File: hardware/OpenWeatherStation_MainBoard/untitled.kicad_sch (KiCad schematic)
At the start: 50 parts, among them Q1 Q_NMOS_GDS, U5 PM8800A, U6 POE13P-33L

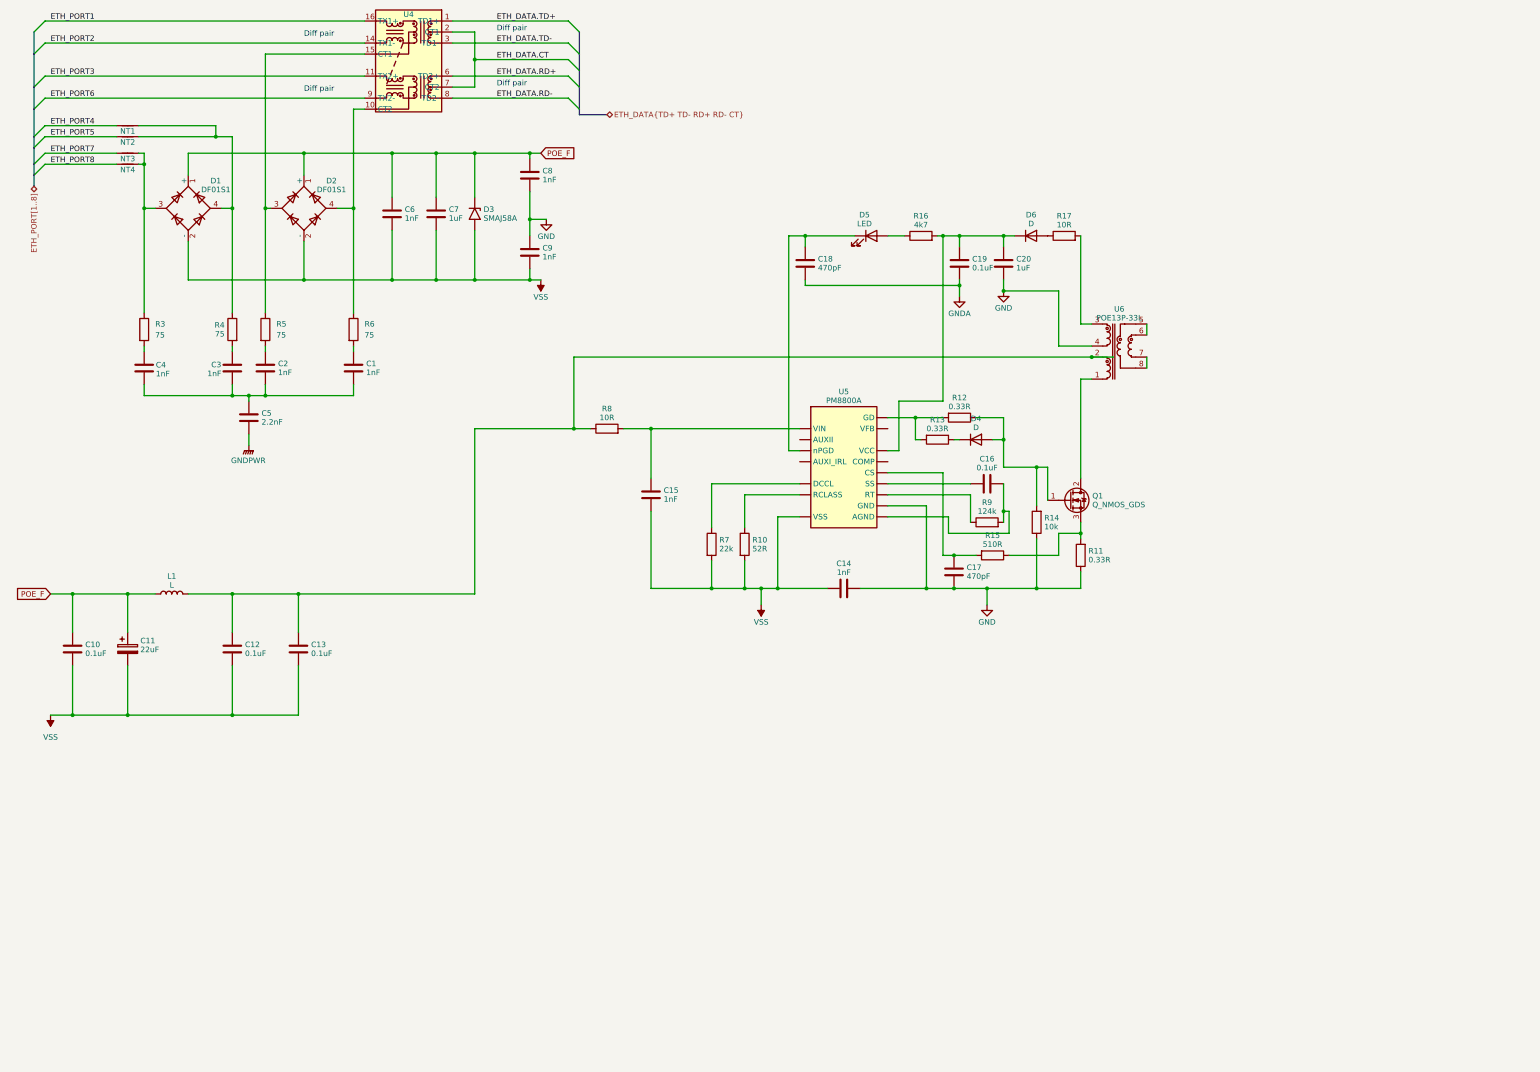
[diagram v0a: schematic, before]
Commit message: poe wip
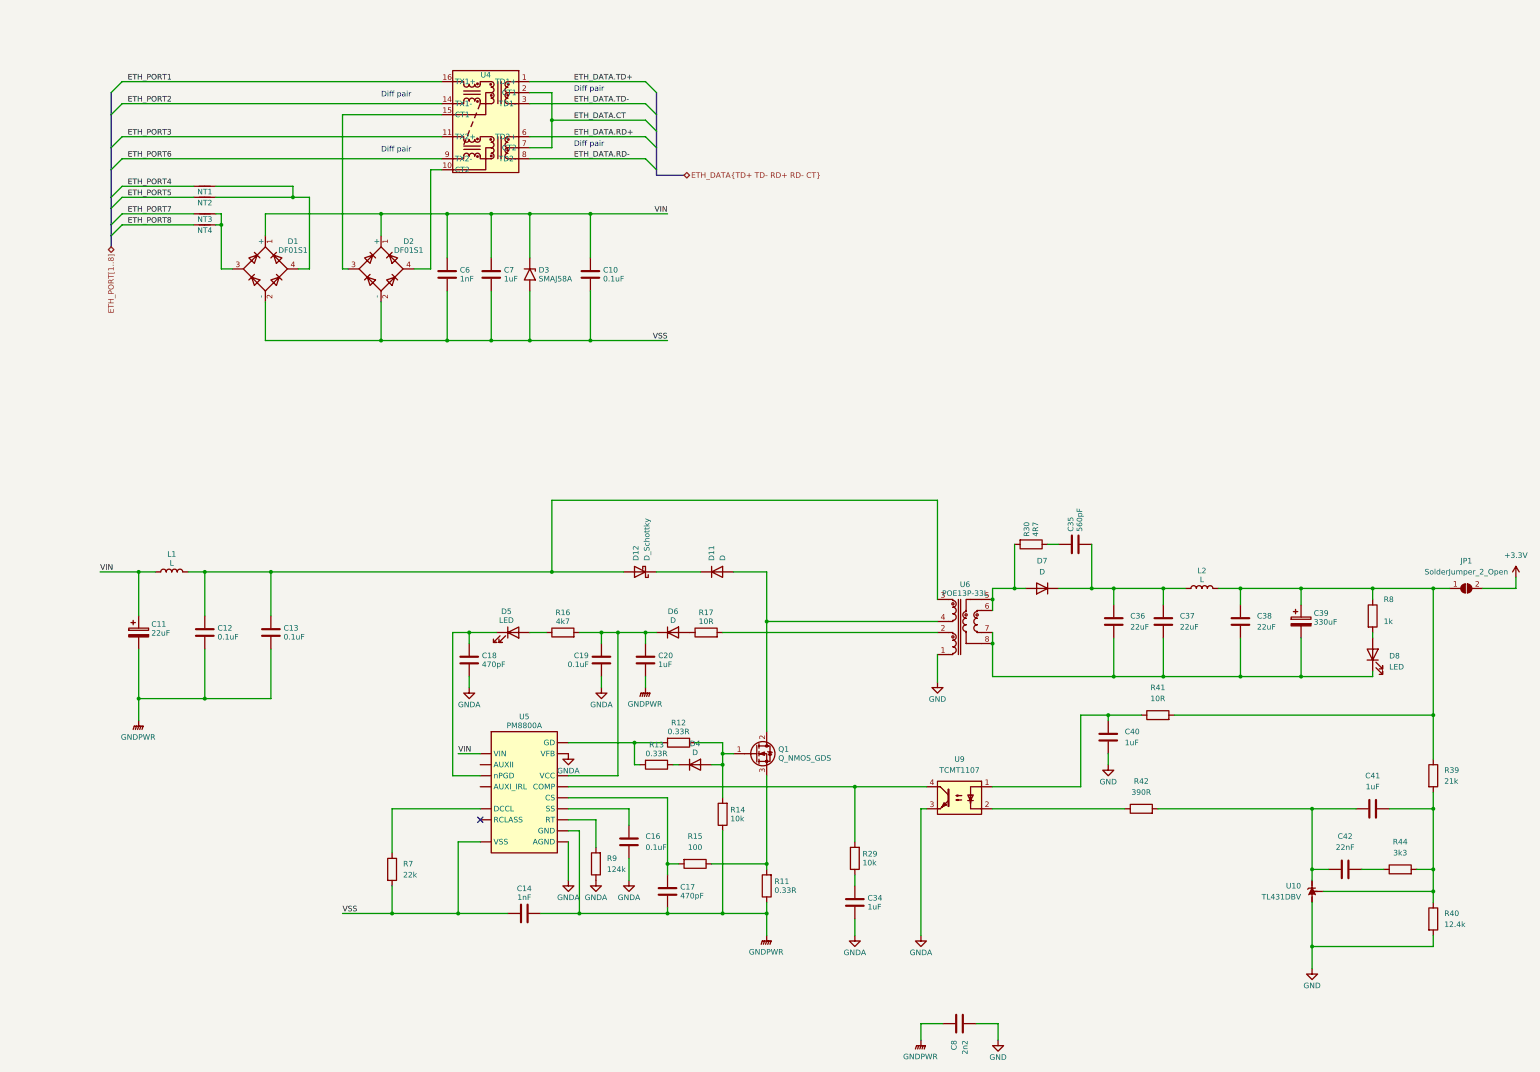
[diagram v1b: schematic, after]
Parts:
- removed C1, C15, C2, C3, C4, C9: 1nF, symbol Device:C
- removed C5: 2.2nF, symbol Device:C
- removed R10: 52R, symbol Device:R
- removed R3, R4, R5, R6: 75, symbol Device:R
- added C34, C40, C41: 1uF, symbol Device:C
- added C35: 560pF, symbol Device:C
- added C36, C37, C38: 22uF, symbol Device:C
- added C39: 330uF, symbol Device:C_Polarized
- added C42: 22nF, symbol Device:C
- added D11, D7: D, symbol Device:D
- added D12: D_Schottky, symbol Device:D_Schottky
- added D8: LED, symbol Device:LED
- added JP1: SolderJumper_2_Open, symbol Jumper:SolderJumper_2_Open
- added L2: L, symbol Device:L
- added R29: 10k, symbol Device:R
- added R30: 4R7, Resistor_SMD:R_1206_3216Metric, symbol Device:R
- added R39: 21k, symbol Device:R
- added R40: 12.4k, symbol Device:R
- added R41: 10R, symbol Device:R
- added R42: 390R, symbol Device:R
- added R44: 3k3, symbol Device:R
- added U10: TL431DBV, Package_TO_SOT_SMD:SOT-23-5, symbol Reference_Voltage:TL431DBV
- added U9: TCMT1107, Package_SO:SOP-4_4.4x2.6mm_P1.27mm, symbol Isolator:TCMT1107
- C8: value 1nF -> 2n2
- R15: value 510R -> 100
- R8: value 10R -> 1k
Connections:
- net GND: now also U6.1, C40.1, R40.2, U10.5 (A); no longer C14.2, C17.2, C20.2, R11.1, R14.1, U5. (nPGD), U6.4
- net GNDA: now also C16.2, R9.1, U5. (nPGD), C34.2, U9.3
- net GNDPWR: now also C11.2, C12.2, C13.2, C14.2, C17.2, C20.2, C8.1, R11.1, R14.1, U5. (nPGD)
- net VSS: no longer C11.2, C12.2, C13.2
- net at C12.1, C13.1, L1.2: now also U6.3, D12.2 (A); no longer R8.1, U6.2
- net at R8.2: now also D8.2 (A); no longer U5. (nPGD)
- net at Q1.2 (D): now also U6.4, D11.2 (A); no longer U6.1
- net at R17.2: now also U6.2; no longer U6.3
- net at U6.5, U6.6: now also D7.2 (A), R30.2
- net at U6.7, U6.8: now also C36.1, C37.1, C38.1, C39.2, D8.1 (K)
- net POE_F renamed VIN
- net VIN: now also U5. (nPGD); no longer C8.1
- new net: D11.1 (K), D12.1 (K)
- new net: R9.2, U5. (nPGD)
- new net: C41.1, R39.2, R40.1, R44.2, U10.4 (REF)
- new net: C40.2, R41.1, U9.1
- new net: C38.2, C39.1, JP1.1 (A), L2.2, R39.1, R41.2, R8.1
- new net: C34.1, R29.1
- new net: R29.2, U5. (nPGD), U9.4
- new net: R42.1, U9.2
- new net: C35.1, R30.1
- new net: C35.2, C36.2, C37.2, D7.1 (K), L2.1
- new net: C42.1, R44.1
- new net: C41.2, C42.2, R42.2, U10.3 (K)
- new net: C16.1, U5. (nPGD)
- new net +3.3V: JP1.2 (B)
- no-connect marks 0 -> 1
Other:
- moved on the sheet: C10, C11, C12, C13, C14, C16, C17, C18, C19, C20, C6, C7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
